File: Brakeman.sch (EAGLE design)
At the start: 9 parts

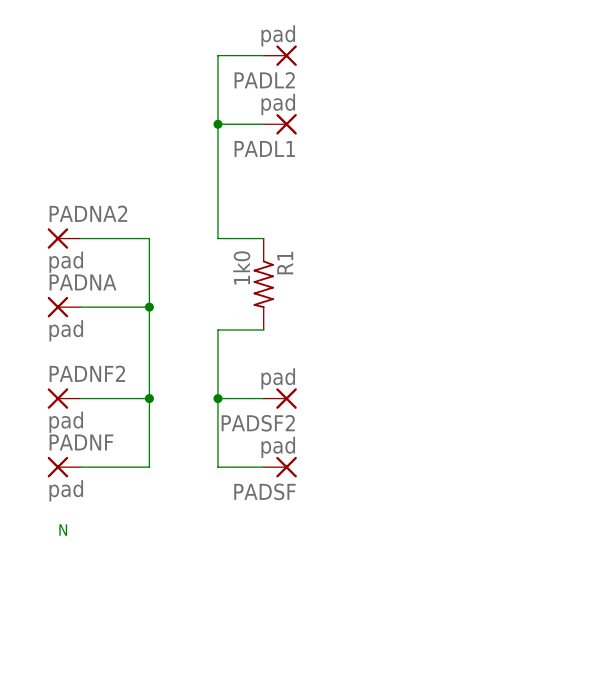
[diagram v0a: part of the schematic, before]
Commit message: Version 2.4
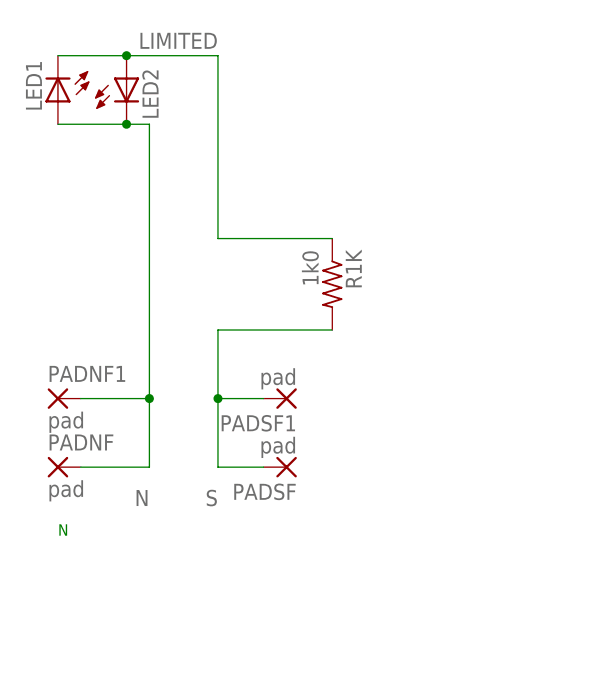
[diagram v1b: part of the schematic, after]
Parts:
- removed PADL1, PADL2, PADNA, PADNA2, PADNF2, PADSF2: pad, wirepad:SMD2
- removed R1: 1k0, resistor:R-US_0204/5
- added LED1, LED2: (no value), SPCoast:LED0603-LED
- added PADNF1, PADSF1: pad, SPCoast:SMD2
- added R1K: 1k0, resistor:R-US_R0603
- PADNF, PADSF: device wirepad:SMD2 -> SPCoast:SMD2
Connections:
- net LIMITED: now also LED1.C, LED2.A, R1K.1; no longer PADL1.P, PADL2.P, R1.1
- net N: now also LED1.A, LED2.C, PADNF1.P; no longer PADNA.P, PADNA2.P, PADNF2.P
- net S: now also PADSF1.P, R1K.2; no longer PADSF2.P, R1.2
